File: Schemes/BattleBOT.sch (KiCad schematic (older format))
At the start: 16 parts

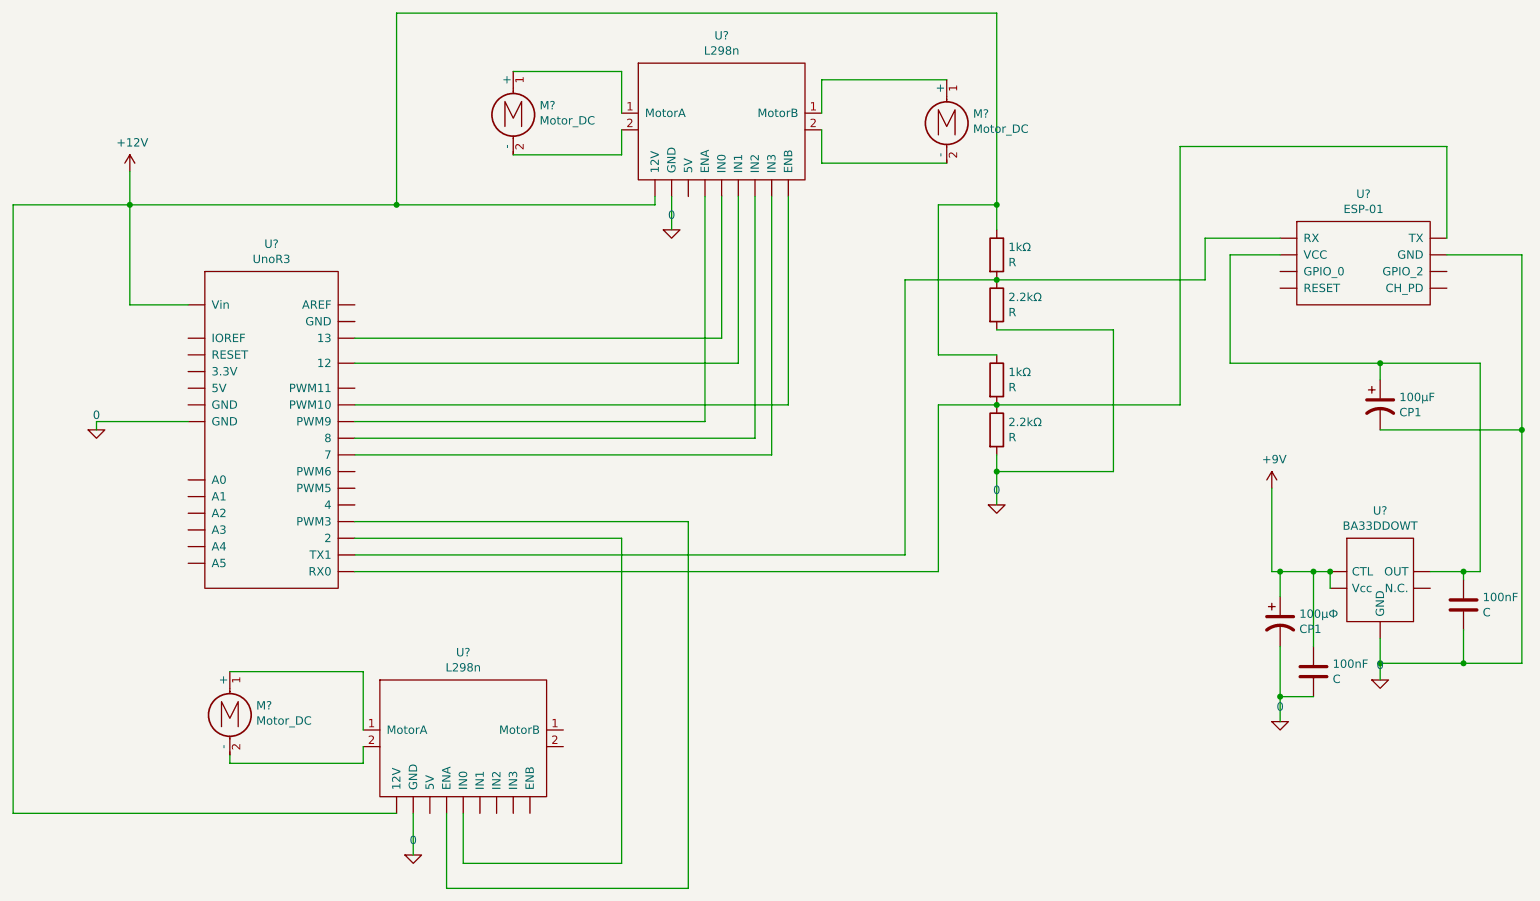
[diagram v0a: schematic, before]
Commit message: make changes to Schemes
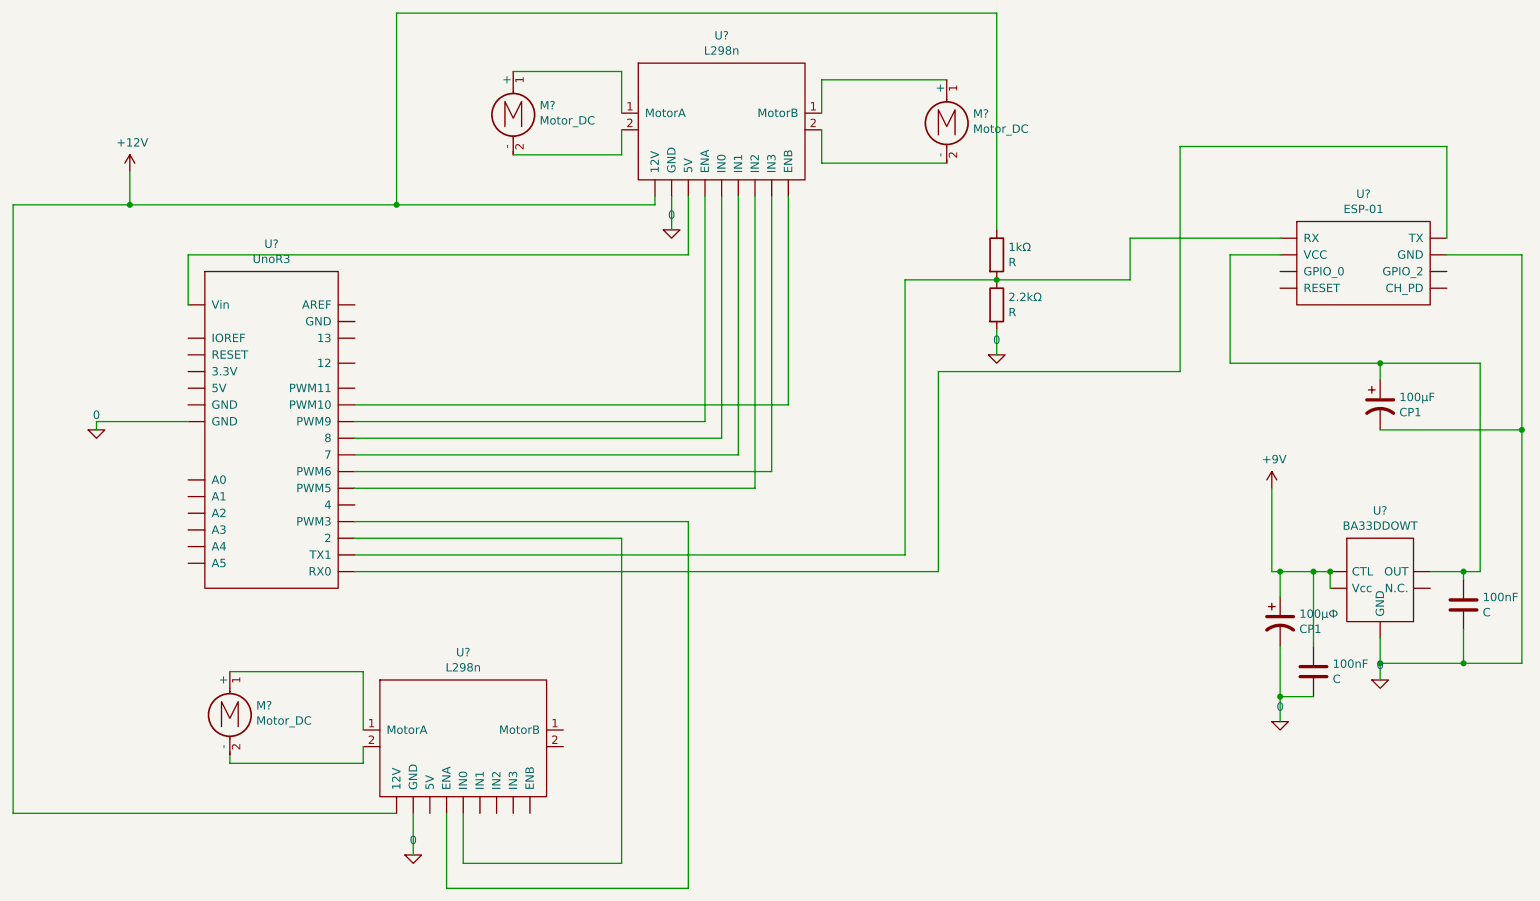
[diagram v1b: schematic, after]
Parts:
- removed 1kΩ, 2.2kΩ: R, symbol Device:R
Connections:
- net +12V: no longer U?.~ (Vin)
- net at U?.1 (MotorB): now also M?.1 (+)
- net at U?.2: now also M?.2 (-)
- new net: U?.~ (IN3), U?.~ (Vin) (x9)
- new net: U?.~ (VCC), U?.~ (Vin)
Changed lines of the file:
@@
 Wire Wire Line
 	2650 1600 2650 1800
-Wire Wire Line
-	2650 2400 3000 2400
 $Comp
 L pspice:0 #GND?
@@
 Connection ~ 2650 1800
 Wire Wire Line
-	2650 1800 2650 2400
-Wire Wire Line
 	2650 1800 4250 1800
 Wire Wire Line
@@
 	3250 5150 3250 5100
 Wire Wire Line
-	4000 2750 6300 2750
-Wire Wire Line
-	6300 2750 6300 1750
-Wire Wire Line
-	6200 1750 6200 2600
-Wire Wire Line
-	6200 2600 4000 2600
-Wire Wire Line
 	4000 3000 6600 3000
 Wire Wire Line
 	6600 3000 6600 1750
-Wire Wire Line
-	6400 1750 6400 3200
-Wire Wire Line
-	6400 3200 4000 3200
-Wire Wire Line
-	6500 1750 6500 3300
-Wire Wire Line
-	6500 3300 4000 3300
 Wire Wire Line
 	4550 5900 6000 5900
@@
 Wire Wire Line
 	10550 1450 10550 2000
-Wire Wire Line
-	9550 2000 9100 2000
 $Comp
 L Device:R 1kΩ
@@
 	1    0    0    -1
 $EndComp
-$Comp
-L Device:R 1kΩ
-U 1 1 5E9473A1
-P 7850 2850
-F 0 "1kΩ" H 7920 2896 50  0000 L CNN
-F 1 "R" H 7920 2805 50  0000 L CNN
-F 2 "" V 7780 2850 50  0001 C CNN
-F 3 "~" H 7850 2850 50  0001 C CNN
-	1    7850 2850
-	1    0    0    -1
-$EndComp
-$Comp
-L Device:R 2.2kΩ
-U 1 1 5E9479C3
-P 7850 3150
-F 0 "2.2kΩ" H 7920 3196 50  0000 L CNN
-F 1 "R" H 7920 3105 50  0000 L CNN
-F 2 "" V 7780 3150 50  0001 C CNN
-F 3 "~" H 7850 3150 50  0001 C CNN
-	1    7850 3150
-	1    0    0    -1
-$EndComp
 Wire Wire Line
 	6100 1750 6100 3100
 Wire Wire Line
 	6100 3100 4000 3100
-Wire Wire Line
-	7850 1950 7850 1800
 Wire Wire Line
 	7850 650  4250 650
@@
 	4250 1800 5800 1800
 Wire Wire Line
-	7850 1800 7500 1800
-Wire Wire Line
-	7500 1800 7500 2700
-Wire Wire Line
-	7500 2700 7850 2700
-Connection ~ 7850 1800
-Wire Wire Line
-	7850 1800 7850 650
-Wire Wire Line
-	7850 2550 8550 2550
-Wire Wire Line
-	8550 2550 8550 3400
-Wire Wire Line
-	8550 3400 7850 3400
-Wire Wire Line
-	7850 3400 7850 3300
-$Comp
-L pspice:0 #GND?
-U 1 1 5EC7A03C
-P 7850 3600
-F 0 "#GND?" H 7850 3500 50  0001 C CNN
-F 1 "0" H 7850 3689 50  0000 C CNN
-F 2 "" H 7850 3600 50  0001 C CNN
-F 3 "~" H 7850 3600 50  0001 C CNN
-	1    7850 3600
-	1    0    0    -1
-$EndComp
-Wire Wire Line
-	7850 3400 7850 3600
-Connection ~ 7850 3400
-Wire Wire Line
-	4000 4000 7500 4000
-Wire Wire Line
-	7500 4000 7500 3000
-Wire Wire Line
-	7500 3000 7850 3000
-Connection ~ 7850 3000
-Wire Wire Line
 	4000 3900 7300 3900
 Wire Wire Line
@@
 Connection ~ 7850 2250
 Wire Wire Line
-	7850 2250 9100 2250
-Wire Wire Line
-	9100 2250 9100 2000
-Wire Wire Line
-	8950 3000 8950 1450
-Wire Wire Line
-	7850 3000 8950 3000
-Wire Wire Line
 	8950 1450 10550 1450
+Wire Wire Line
+	6000 1750 6000 2100
+Wire Wire Line
+	6000 2100 3000 2100
+Wire Wire Line
+	3000 2100 3000 2400
+Wire Wire Line
+	7850 650  7850 1950
+$Comp
+L pspice:0 #GND?
+U 1 1 5EC82388
+P 7850 2700
+F 0 "#GND?" H 7850 2600 50  0001 C CNN
+F 1 "0" H 7850 2789 50  0000 C CNN
+F 2 "" H 7850 2700 50  0001 C CNN
+F 3 "~" H 7850 2700 50  0001 C CNN
+	1    7850 2700
+	1    0    0    -1
+$EndComp
+Wire Wire Line
+	7850 2550 7850 2700
+Wire Wire Line
+	4000 4000 7500 4000
+Wire Wire Line
+	7500 4000 7500 2800
+Wire Wire Line
+	7500 2800 8950 2800
+Wire Wire Line
+	8950 2800 8950 1450
+Wire Wire Line
+	8650 2250 8650 2000
+Wire Wire Line
+	8650 2000 9550 2000
+Wire Wire Line
+	7850 2250 8650 2250
+Wire Wire Line
+	4000 3200 6200 3200
+Wire Wire Line
+	6200 3200 6200 1750
+Wire Wire Line
+	4000 3300 6300 3300
+Wire Wire Line
+	6300 3300 6300 1750
+Wire Wire Line
+	4000 3400 6500 3400
+Wire Wire Line
+	6500 3400 6500 1750
+Wire Wire Line
+	4000 3500 6400 3500
+Wire Wire Line
+	6400 3500 6400 1750
 $EndSCHEMATC
